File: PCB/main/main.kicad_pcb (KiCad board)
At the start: 2 copper layers, 4 parts, among them J1 Conn_01x33_Female, J2 Conn_01x33_Female, J3 Conn_01x33_Female, J4 Conn_01x33_Female

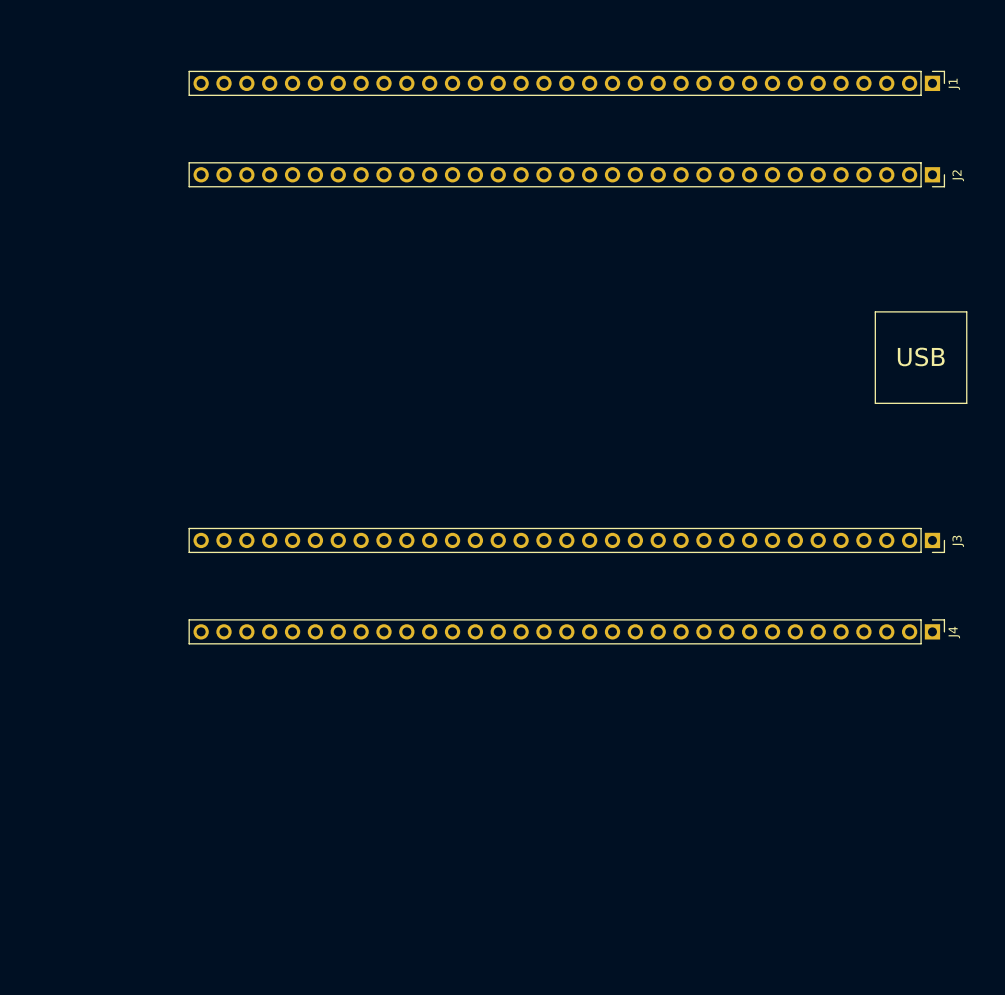
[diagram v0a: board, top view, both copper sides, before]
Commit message: Design PCB
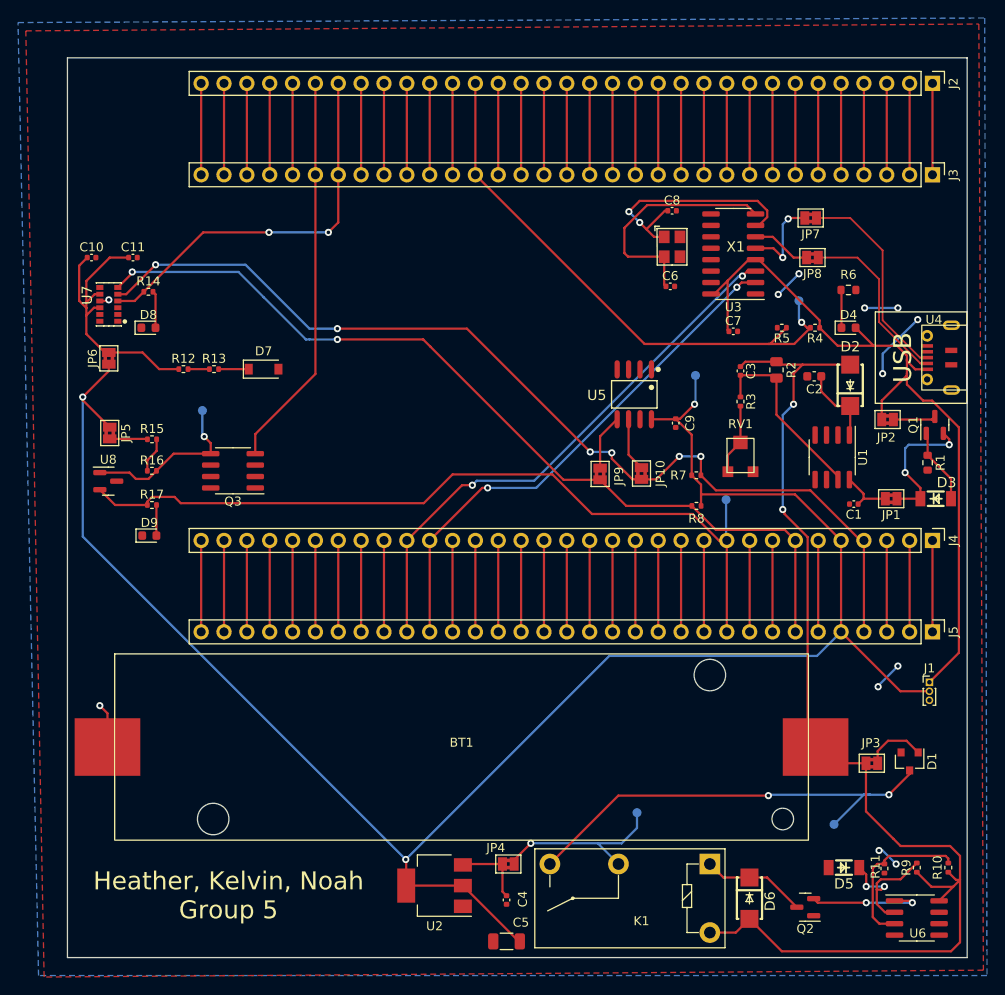
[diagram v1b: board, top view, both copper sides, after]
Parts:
- added BT1: 18650, Footprint_EEE3088F:18650_Holder, F.Cu at (128.0, 139.8)
- added C1: 0.1uF, Capacitor_SMD:C_0402_1005Metric, F.Cu at (171.6, 112.8)
- added C10: 100nF, Capacitor_SMD:C_0402_1005Metric, F.Cu at (86.9, 85.4)
- added C11: 4.7nF, Capacitor_SMD:C_0402_1005Metric, F.Cu at (91.5, 85.4)
- added C2: 22uF, Capacitor_SMD:C_0603_1608Metric, F.Cu at (167.2, 98.6)
- added C3: 330pF, Capacitor_SMD:C_0402_1005Metric, F.Cu at (159.0, 98.0)
- added C4: 0.1uF, Capacitor_SMD:C_0402_1005Metric, F.Cu at (133.0, 156.8)
- added C5: 100uF, Capacitor_SMD:C_1206_3216Metric, F.Cu at (133.0, 161.4)
- added C6: 33pF, Capacitor_SMD:C_0402_1005Metric, F.Cu at (151.2, 88.6)
- added C7: 10nF, Capacitor_SMD:C_0402_1005Metric, F.Cu at (158.2, 93.6)
- added C8: 33pF, Capacitor_SMD:C_0402_1005Metric, F.Cu at (151.4, 80.2)
- added C9: 0.1uF, Capacitor_SMD:C_0402_1005Metric, F.Cu at (151.8, 103.8)
- added D1: BAT54S, Diode_SMD:D_SOT-23_ANK, F.Cu at (177.8, 141.4)
- added D2: DIODE, Footprint_EEE3088F:DO-214AC_L4.3-W2.7-LS5.3-RD, F.Cu at (171.2, 99.6)
- added D3: ZMM5V1-M, Footprint_EEE3088F:LL-34_L3.5-W1.5-RD, F.Cu at (180.7, 112.2)
- added D4: LED, LED_SMD:LED_0603_1608Metric, F.Cu at (171.0, 93.2)
- added D5: ZMM4V7-M, Footprint_EEE3088F:LL-34_L3.5-W1.5-RD, F.Cu at (170.5, 153.2)
- added D6: DIODE, Footprint_EEE3088F:DO-214AC_L4.3-W2.7-LS5.3-RD, F.Cu at (160.0, 156.6)
- added D7: BZT52C3V0, Diode_SMD:D_SOD-123, F.Cu at (106.0, 97.8)
- added D8: LED, LED_SMD:LED_0603_1608Metric, F.Cu at (93.2, 93.2)
- added D9: LED, LED_SMD:LED_0603_1608Metric, F.Cu at (93.3, 116.3)
- added J1: Conn_01x03_Female, Connector_PinHeader_1.00mm:PinHeader_1x03_P1.00mm_Vertical, F.Cu at (180.0, 132.6)
- added JP1: SolderJumper_2_Bridged, Jumper:SolderJumper-2_P1.3mm_Bridged2Bar_Pad1.0x1.5mm, F.Cu at (175.8, 112.2)
- added JP10: SolderJumper_2_Bridged, Jumper:SolderJumper-2_P1.3mm_Bridged2Bar_Pad1.0x1.5mm, F.Cu at (148.0, 109.4)
- added JP2: SolderJumper_2_Bridged, Jumper:SolderJumper-2_P1.3mm_Bridged2Bar_Pad1.0x1.5mm, F.Cu at (175.3, 103.4)
- added JP3: SolderJumper_2_Bridged, Jumper:SolderJumper-2_P1.3mm_Bridged2Bar_Pad1.0x1.5mm, F.Cu at (173.6, 141.6)
- added JP4: SolderJumper_2_Bridged, Jumper:SolderJumper-2_P1.3mm_Bridged2Bar_Pad1.0x1.5mm, F.Cu at (133.2, 152.8)
- added JP5: SolderJumper_2_Bridged, Jumper:SolderJumper-2_P1.3mm_Bridged2Bar_Pad1.0x1.5mm, F.Cu at (88.9, 104.9)
- added JP6: SolderJumper_2_Bridged, Jumper:SolderJumper-2_P1.3mm_Bridged2Bar_Pad1.0x1.5mm, F.Cu at (88.8, 96.6)
- added JP7: SolderJumper_2_Bridged, Jumper:SolderJumper-2_P1.3mm_Bridged2Bar_Pad1.0x1.5mm, F.Cu at (166.8, 81.0)
- added JP8: SolderJumper_2_Bridged, Jumper:SolderJumper-2_P1.3mm_Bridged2Bar_Pad1.0x1.5mm, F.Cu at (167.0, 85.4)
- added JP9: SolderJumper_2_Bridged, Jumper:SolderJumper-2_P1.3mm_Bridged2Bar_Pad1.0x1.5mm, F.Cu at (143.4, 109.5)
- added K1: ADW11, Relay_THT:Relay_SPST_Omron-G5Q-1A, F.Cu at (155.6, 152.8)
- added Q1: AO3401A, Package_TO_SOT_SMD:SOT-23, F.Cu at (180.6, 104.0)
- added Q2: 2N3904, Package_TO_SOT_SMD:SOT-23, F.Cu at (166.2, 157.6)
- added Q3: FDS6690A, Package_SO:SOIC-8_3.9x4.9mm_P1.27mm, F.Cu at (102.6, 109.1)
- added R1: 100, Resistor_SMD:R_0603_1608Metric, F.Cu at (179.8, 108.2)
- added R10: 1k, Resistor_SMD:R_0402_1005Metric, F.Cu at (182.1, 153.2)
- added R11: 100k, Resistor_SMD:R_0402_1005Metric, F.Cu at (175.0, 153.3)
- added R12: 330, Resistor_SMD:R_0402_1005Metric, F.Cu at (97.1, 97.8)
- added R13: 330, Resistor_SMD:R_0402_1005Metric, F.Cu at (100.5, 97.8)
- added R14: 10k, Resistor_SMD:R_0402_1005Metric, F.Cu at (93.2, 89.2)
- added R15: 330, Resistor_SMD:R_0402_1005Metric, F.Cu at (93.6, 105.6)
- added R16: 220, Resistor_SMD:R_0402_1005Metric, F.Cu at (93.6, 109.1)
- added R17: 10k, Resistor_SMD:R_0402_1005Metric, F.Cu at (93.6, 112.9)
- added R2: 2M, Resistor_SMD:R_0805_2012Metric, F.Cu at (163.0, 97.9)
- added R3: 806K, Resistor_SMD:R_0402_1005Metric, F.Cu at (159.0, 101.4)
- added R4: 2.7k, Resistor_SMD:R_0402_1005Metric, F.Cu at (167.3, 93.2)
- added R5: 4.7k, Resistor_SMD:R_0402_1005Metric, F.Cu at (163.6, 93.2)
- added R6: 82, Resistor_SMD:R_0603_1608Metric, F.Cu at (171.0, 89.0)
- added R7: 10k, Resistor_SMD:R_0402_1005Metric, F.Cu at (154.1, 109.6)
- added R8: 10k, Resistor_SMD:R_0402_1005Metric, F.Cu at (154.1, 113.0)
- added R9: 150, Resistor_SMD:R_0402_1005Metric, F.Cu at (178.6, 153.2)
- added RV1: 50K, Footprint_EEE3088F:VG039NCHXTB503, F.Cu at (159.0, 107.4)
- added TP1: TestPoint, TestPoint:TestPoint_Pad_D1.0mm, B.Cu at (169.4, 148.4)
- added TP2: TestPoint, TestPoint:TestPoint_Pad_D1.0mm, B.Cu at (154.0, 98.5)
- added TP3: TestPoint, TestPoint:TestPoint_Pad_D1.0mm, B.Cu at (165.5, 90.2)
- added TP4: TestPoint, TestPoint:TestPoint_Pad_D1.0mm, B.Cu at (147.5, 147.1)
- added TP5: TestPoint, TestPoint:TestPoint_Pad_D1.0mm, B.Cu at (99.2, 102.4)
- added TP6: TestPoint, TestPoint:TestPoint_Pad_D1.0mm, B.Cu at (157.4, 112.3)
- added U1: LP2951-33DR, Package_SO:SOIC-8_3.9x4.9mm_P1.27mm, F.Cu at (169.2, 107.6)
- added U2: AMS1117, Package_TO_SOT_SMD:SOT-223-3_TabPin2, F.Cu at (125.0, 155.2)
- added U3: CH340G, Package_SO:SOIC-16_3.9x9.9mm_P1.27mm, F.Cu at (158.2, 85.0)
- added U4: USB_Micro_B, Footprint_EEE3088F:C404969_Micro_USB, F.Cu at (184.2, 96.5)
- added U5: AT24C256C-SSHL-T, Footprint_EEE3088F:SOIC-8_L4.9-W3.9-P1.27-LS6.0-BL, F.Cu at (147.2, 100.6)
- added U6: LM358DR2G, Package_SO:SOIC-8_3.9x4.9mm_P1.27mm, F.Cu at (178.6, 158.8)
- added U7: VL6180XV0NR_1, Footprint_EEE3088F:LGA-12_L4.8-W2.8-P0.75-BL, F.Cu at (88.8, 90.6)
- added U8: MCP9700T-ETT, Package_TO_SOT_SMD:SOT-23, F.Cu at (88.7, 110.2)
- added X1: 12MHz Crystal, Footprint_EEE3088F:OSC-SMD_4P-L3.2-W2.5-BL, F.Cu at (151.4, 84.2)
- J3: renamed from J2; footprint Connector_PinSocket_2.54mm:PinSocket_1x33_P2.54mm_Vertical -> Connector_PinHeader_2.54mm:PinHeader_1x33_P2.54mm_Vertical
- J4: renamed from J3; footprint Connector_PinSocket_2.54mm:PinSocket_1x33_P2.54mm_Vertical -> Connector_PinHeader_2.54mm:PinHeader_1x33_P2.54mm_Vertical
- renumbered J1 to J2, J4 to J5
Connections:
- net +3V0 renamed /+3V0
- net +5V renamed /+5V
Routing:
- net VDD: track 0.00 -> 212.7 mm, vias 0 -> 3
- net /Power/Battery +: track 0.00 -> 131.3 mm, vias 0 -> 2
- net /PB8: track 0.00 -> 110.9 mm, vias 0 -> 6
- net /PB7: track 0.00 -> 98.6 mm, vias 0 -> 2
- net /PB4: track 0.00 -> 90.4 mm
- net /microcontroller_interfacing/+5V: track 0.00 -> 86.5 mm
- net GND: track 0.00 -> 77.1 mm, vias 0 -> 12
- net /PA4: track 0.00 -> 62.4 mm, vias 0 -> 1
- net /PA9: track 0.00 -> 61.3 mm, vias 0 -> 2
- net /PA10: track 0.00 -> 58.2 mm, vias 0 -> 2
- net /Power/+5V (REVERSE PROTECTED): track 0.00 -> 49.9 mm, vias 0 -> 2
- net /PB1: track 0.00 -> 43.9 mm
- net /PB0: track 0.00 -> 43.6 mm, vias 0 -> 2
- net /Sensing/Proximity_Sensor/VCC: track 0.00 -> 33.6 mm
- net Net-(C8-Pad1): track 0.00 -> 27.0 mm, vias 0 -> 2
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- added copper zone on B.Cu, net (none)
- added copper zone on F.Cu, net GND
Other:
- board outline added: 100 x 100 mm
- board text added: "Heather, Kelvin, Noah Group 5"
